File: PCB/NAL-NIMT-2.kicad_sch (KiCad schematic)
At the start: 27 parts

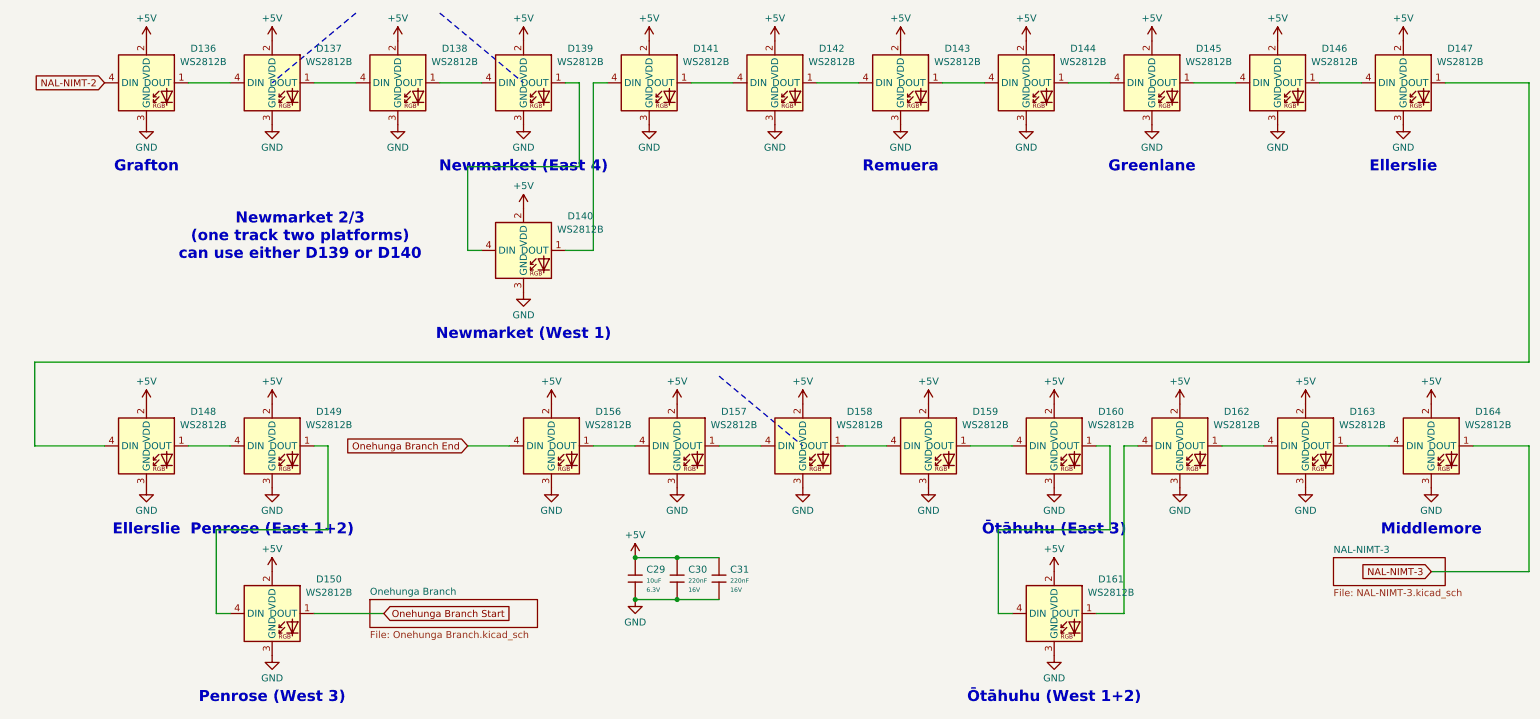
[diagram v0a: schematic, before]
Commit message: Final tweaks for V1.0.0
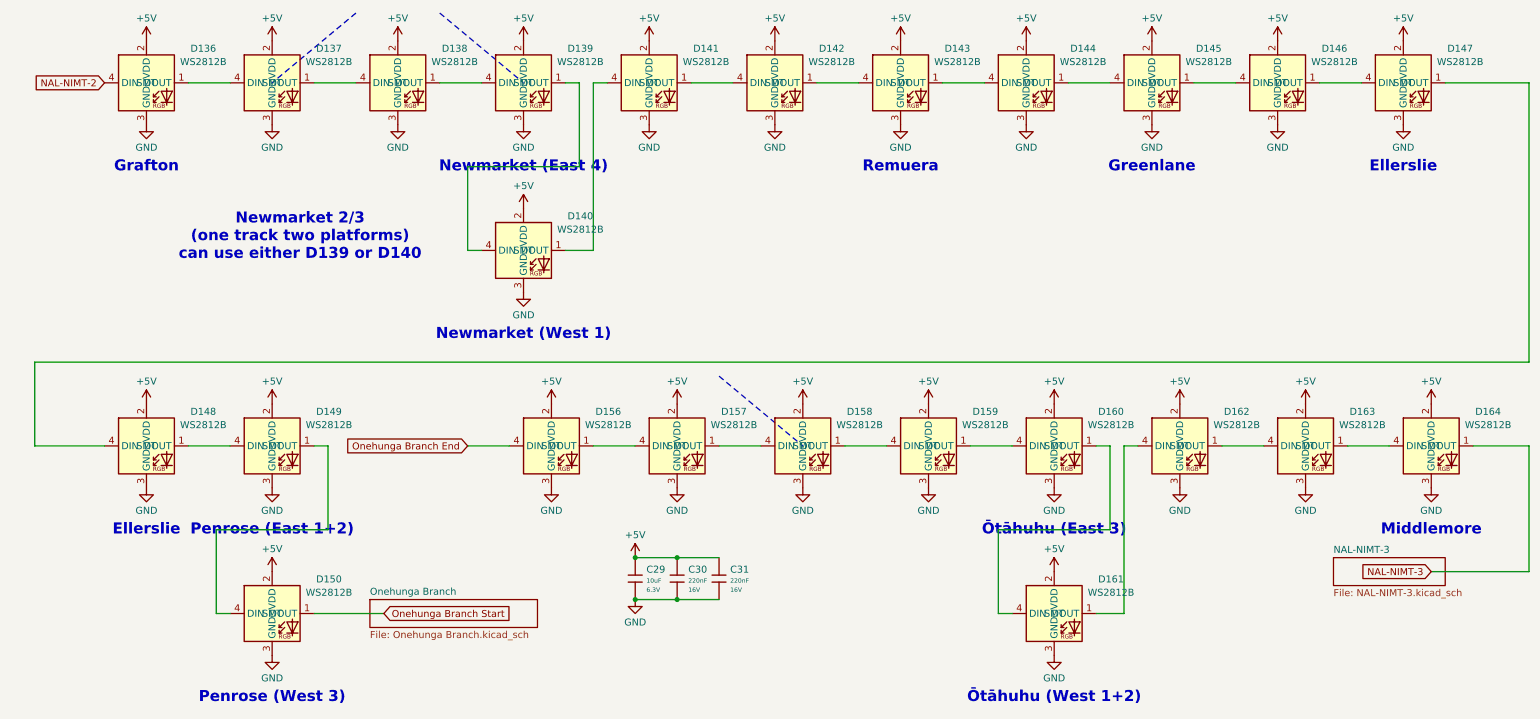
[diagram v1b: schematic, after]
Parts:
- D136, D137, D138, D139, D140, D141, D142, D143, D144, D145, D146, D147, D148, D149, D150, D156, D157, D158, D159, D160, D161, D162, D163, D164: Manufacturer (none) -> XINGLIGHT; Part (none) -> XL-1615RGBC-WS2812B; Process (none) -> SMT
